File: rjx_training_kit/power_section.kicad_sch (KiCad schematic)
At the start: 12 parts, among them J1 Barrel_Jack_Switch, J2 USB_B_Mini, SW1 SW_SPDT, U6 MPM3610GQV-P

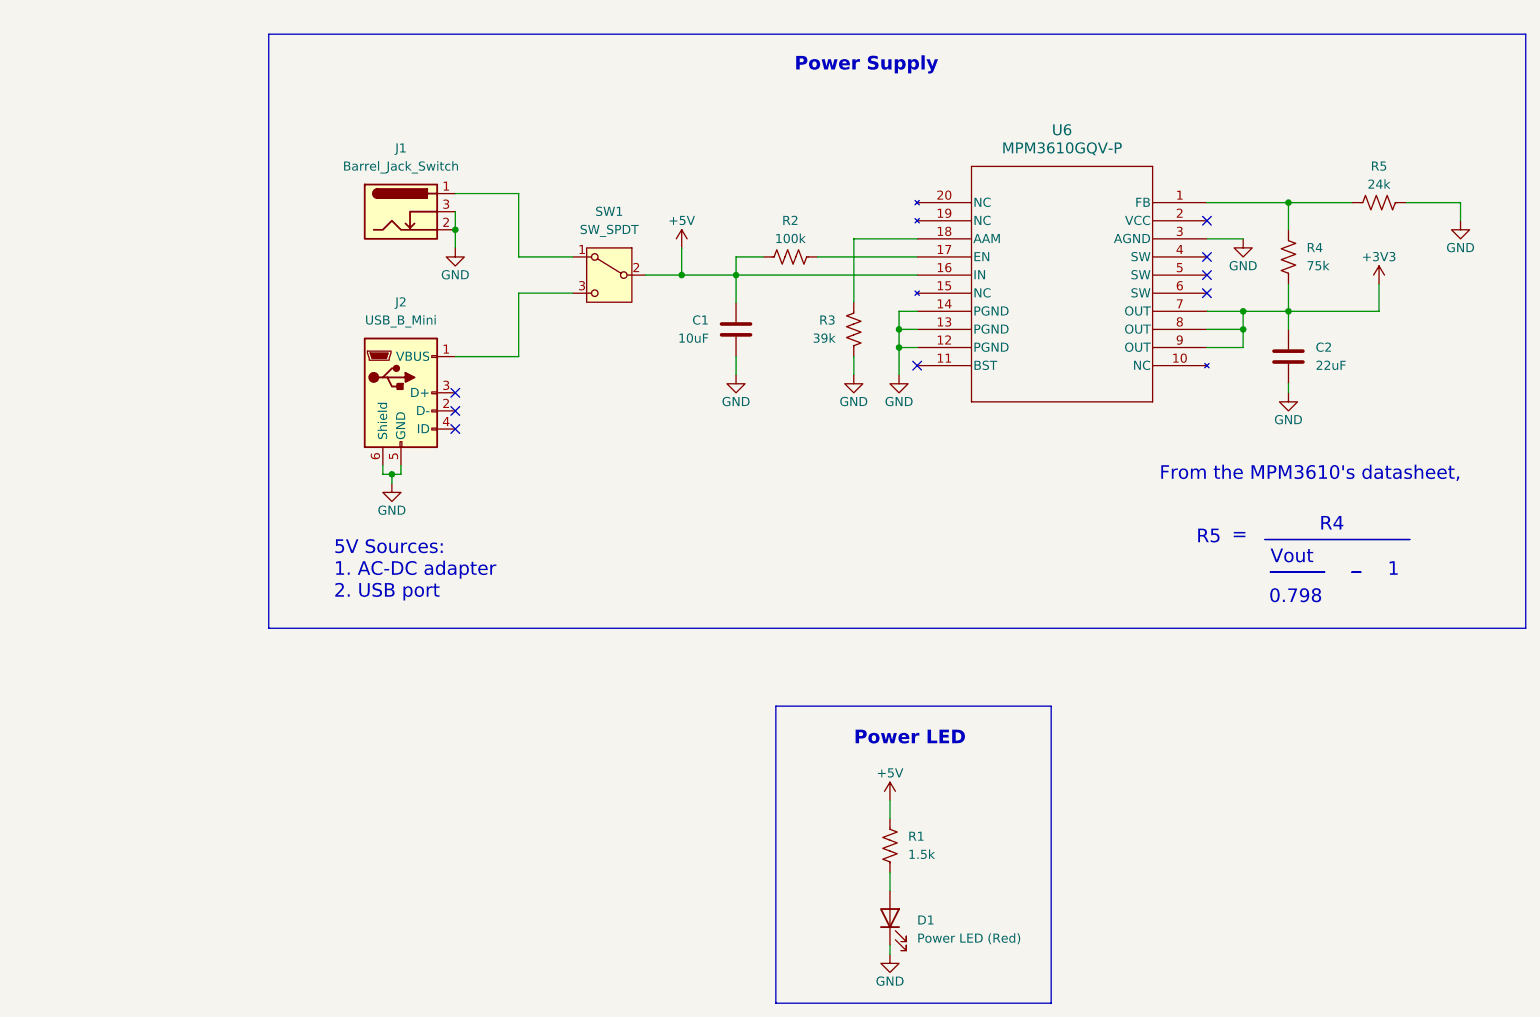
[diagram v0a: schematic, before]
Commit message: Update
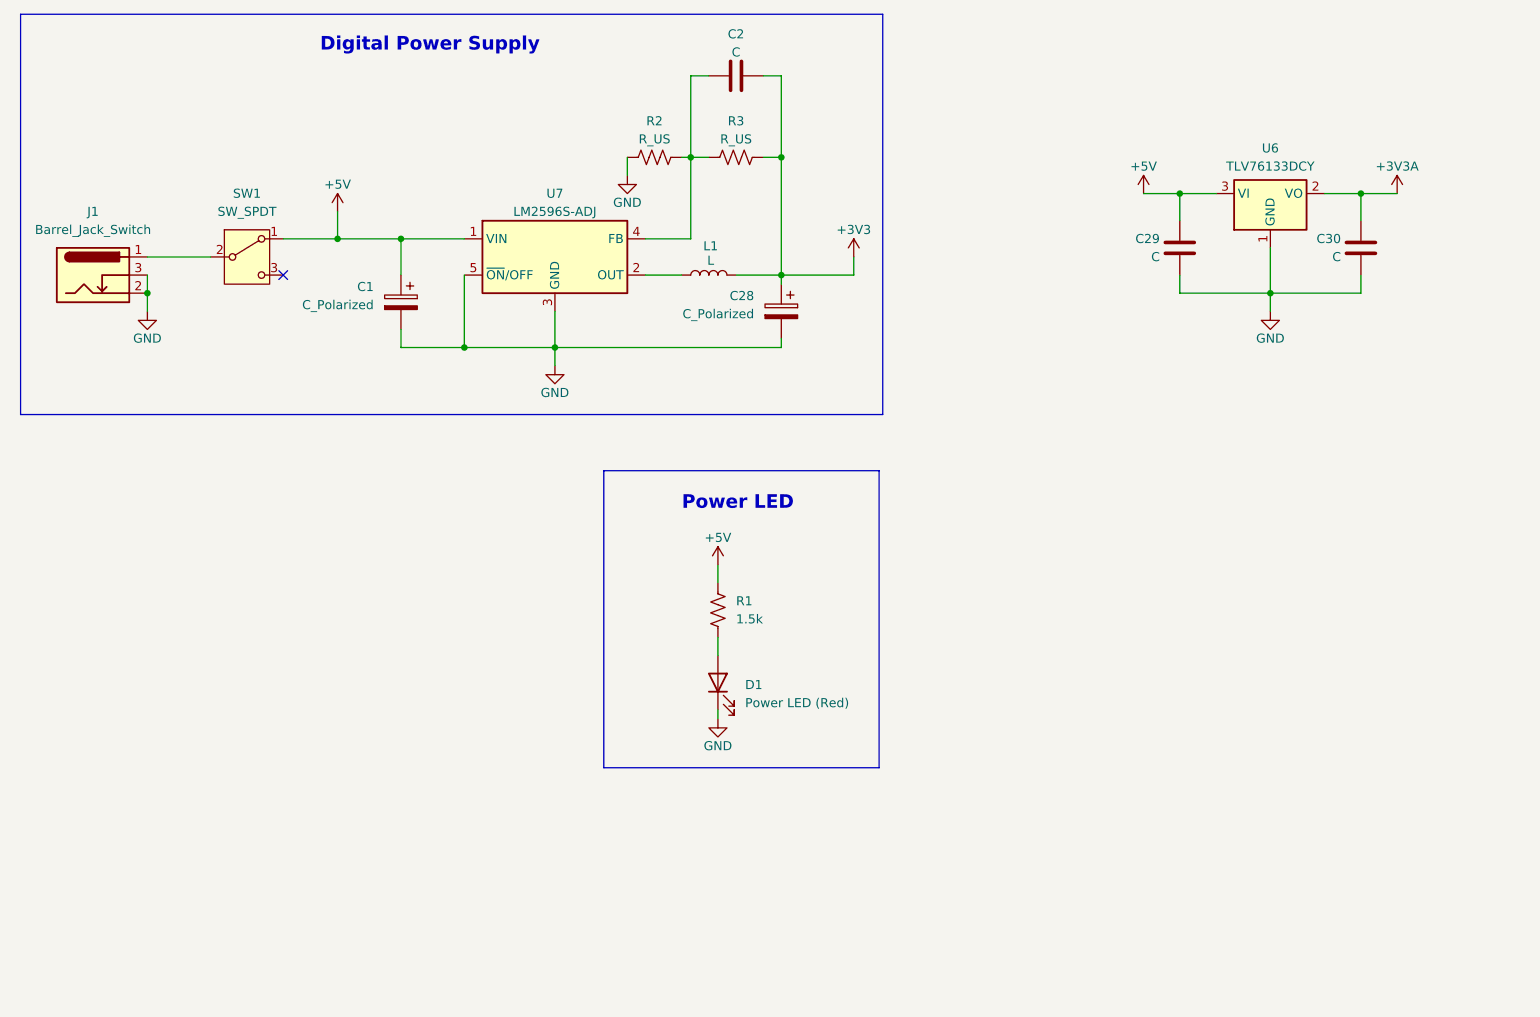
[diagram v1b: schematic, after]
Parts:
- removed C1: 10uF, symbol Device:C
- removed J2: USB_B_Mini, symbol Connector:USB_B_Mini
- removed R4: 75k, symbol Device:R_US
- removed R5: 24k, symbol Device:R_US
- removed U6: MPM3610GQV-P, QFN3p0x5p0x1p6_MPM3610_MNP, symbol mpm3610:MPM3610GQV-P
- added C1, C28: C_Polarized, symbol Device:C_Polarized
- added C29, C30: C, symbol Device:C
- added L1: L, symbol Device:L
- added U6: TLV76133DCY, Package_TO_SOT_SMD:SOT-223-3_TabPin2, symbol Regulator_Linear:TLV76133DCY
- added U7: LM2596S-ADJ, Package_TO_SOT_SMD:TO-263-5_TabPin3, symbol Regulator_Switching:LM2596S-ADJ
- C2: value 22uF -> C
- R2: value 100k -> R_US
- R3: value 39k -> R_US
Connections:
- net +3V3: now also C2.2, R3.2, C28.1, L1.1; no longer C2.1
- net +5V: now also SW1.1 (A), C1.1, C29.1, U6.3 (VI), U7.1 (VIN); no longer R2.2, SW1.2 (B)
- net GND: now also R2.1, C1.2, C28.2, C29.2, C30.2, U6.1 (GND), U7.3 (GND), U7.5 (~{ON}/OFF); no longer C2.2, R3.1
- net at J1.1: now also SW1.2 (B); no longer SW1.1 (A)
- new net: C2.1, R2.2, R3.1, U7.4 (FB)
- new net: L1.2, U7.2 (OUT)
- new net +3V3A: C30.1, U6.2 (VO)
- no-connect marks 8 -> 1
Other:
- note added: "Digital Power Supply"
- note removed: "0.798"
- note removed: "1"
- note removed: "5V Sources: 1. AC-DC adapter 2. USB port"
- note removed: "="
- note removed: "From the MPM3610's datasheet,"
- note removed: "Power Supply"
- note removed: "R4"
- note removed: "R5"
- note removed: "Vout"
- moved on the sheet: D1, J1, R1, SW1
